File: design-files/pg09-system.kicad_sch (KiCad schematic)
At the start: 34 parts, among them J101 Front Panel, SW201 NMI, SW201 Reset, U101 MC6809E, U102 GAL22V10, U103 74AHCT245, U104 74AHCT245, U105 74AHCT245, U106 GAL22V10, U203 DS1813

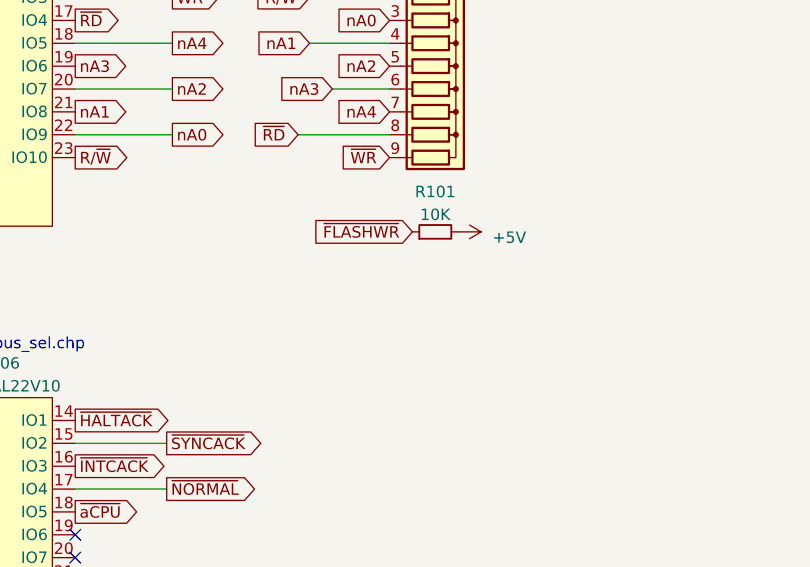
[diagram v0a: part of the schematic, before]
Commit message: Make sure FLASHWREN always has a valid value by pulling it to GND.
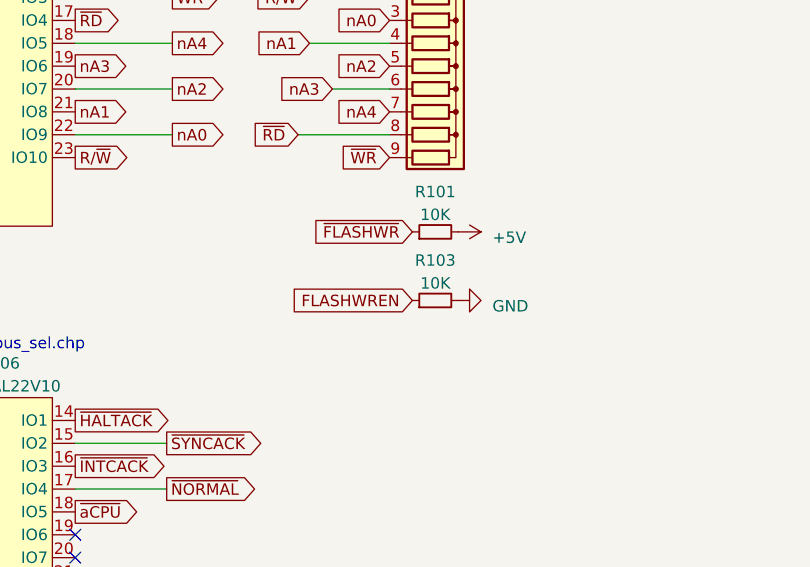
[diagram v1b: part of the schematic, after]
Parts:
- added R103: 10K, Resistor_THT:R_Axial_DIN0207_L6.3mm_D2.5mm_P7.62mm_Horizontal, symbol Device:R_Small
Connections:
- net FLASHWREN: now also R103.1
- net GND: now also R103.2
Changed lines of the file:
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@@
+    )
+  )
+  (global_label "FLASHWREN" (shape input) (at 321.31 163.83 180) (fields_autoplaced)
+    (effects (font (size 1.27 1.27)) (justify right))
+    (property "Intersheetrefs" "${INTERSHEET_REFS}" (at 307.458 163.83 0)
+      (effects (font (size 1.27 1.27)) (justify right) hide)
     )
   )
@@
     )
   )
+  (symbol (lib_id "power:GND") (at 326.39 163.83 90) (unit 1)
+    (in_bom yes) (on_board yes) (dnp no) (fields_autoplaced)
+    (property "Reference" "#PWR0131" (at 332.74 163.83 0)
+      (effects (font (size 1.27 1.27)) hide)
+    )
+    (property "Value" "GND" (at 330.2 164.465 90)
+      (effects (font (size 1.27 1.27)) (justify right))
+    )
+    (property "Footprint" "" (at 326.39 163.83 0)
+      (effects (font (size 1.27 1.27)) hide)
+    )
+    (property "Datasheet" "" (at 326.39 163.83 0)
+      (effects (font (size 1.27 1.27)) hide)
+    )
+    (pin "1")
+    (instances
+      (project "pg09-system"
+        (path "/44572023-3621-4b3a-bd53-c3b2b3f42871"
+          (reference "#PWR0131") (unit 1)
+        )
+      )
+    )
+  )
   (symbol (lib_id "power:GND") (at 116.84 183.388 0) (unit 1)
     (in_bom yes) (on_board yes) (dnp no) (fields_autoplaced)
@@
         )
       )
+    )
+  )
+  (symbol (lib_id "Device:R_Small") (at 323.85 163.83 90) (unit 1)
+    (in_bom yes) (on_board yes) (dnp no) (fields_autoplaced)
+    (property "Reference" "R103" (at 323.85 159.385 90)
+      (effects (font (size 1.27 1.27)))
+    )
+    (property "Value" "10K" (at 323.85 161.925 90)
+      (effects (font (size 1.27 1.27)))
+    )
+    (property "Footprint" "Resistor_THT:R_Axial_DIN0207_L6.3mm_D2.5mm_P7.62mm_Horizontal" (at 323.85 163.83 0)
+      (effects (font (size 1.27 1.27)) hide)
+    )
+    (property "Datasheet" "~" (at 323.85 163.83 0)
+      (effects (font (size 1.27 1.27)) hide)
+    )
+    (pin "1")
+    (pin "2")
+    (instances
+      (project "pg09-system"
+        (path "/44572023-3621-4b3a-bd53-c3b2b3f42871"
+          (reference "R103") (unit 1)
+        )
+      )

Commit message: Revert "Make sure FLASHWREN always has a valid value by pulling it to GND."
This is actually counter-productive due to the internal pull-up on the
GAL inputs.

This reverts commit e5d063032c780da183b0786b1f57988b4be9d05e.
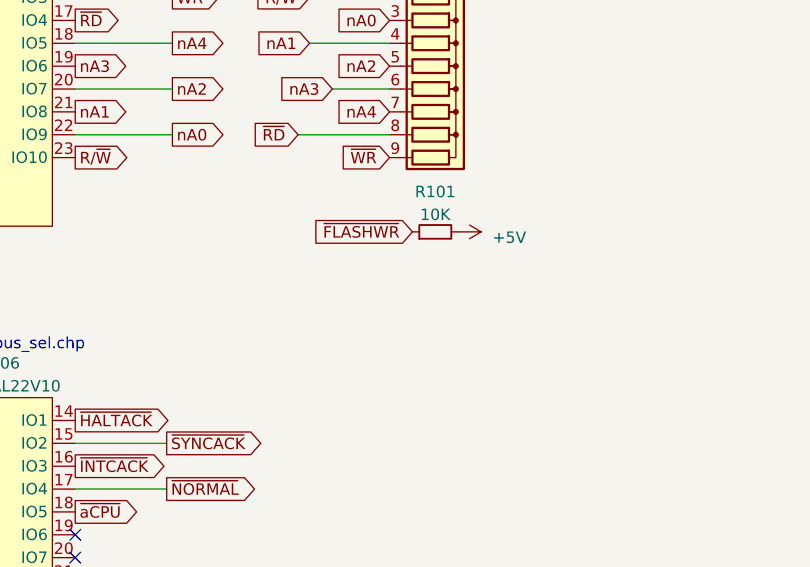
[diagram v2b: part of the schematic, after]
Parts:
- removed R103: 10K, Resistor_THT:R_Axial_DIN0207_L6.3mm_D2.5mm_P7.62mm_Horizontal, symbol Device:R_Small
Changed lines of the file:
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@@
-    )
-  )
-  (global_label "FLASHWREN" (shape input) (at 321.31 163.83 180) (fields_autoplaced)
-    (effects (font (size 1.27 1.27)) (justify right))
-    (property "Intersheetrefs" "${INTERSHEET_REFS}" (at 307.458 163.83 0)
-      (effects (font (size 1.27 1.27)) (justify right) hide)
     )
   )
@@
     )
   )
-  (symbol (lib_id "power:GND") (at 326.39 163.83 90) (unit 1)
-    (in_bom yes) (on_board yes) (dnp no) (fields_autoplaced)
-    (property "Reference" "#PWR0131" (at 332.74 163.83 0)
-      (effects (font (size 1.27 1.27)) hide)
-    )
-    (property "Value" "GND" (at 330.2 164.465 90)
-      (effects (font (size 1.27 1.27)) (justify right))
-    )
-    (property "Footprint" "" (at 326.39 163.83 0)
-      (effects (font (size 1.27 1.27)) hide)
-    )
-    (property "Datasheet" "" (at 326.39 163.83 0)
-      (effects (font (size 1.27 1.27)) hide)
-    )
-    (pin "1")
-    (instances
-      (project "pg09-system"
-        (path "/44572023-3621-4b3a-bd53-c3b2b3f42871"
-          (reference "#PWR0131") (unit 1)
-        )
-      )
-    )
-  )
   (symbol (lib_id "power:GND") (at 116.84 183.388 0) (unit 1)
     (in_bom yes) (on_board yes) (dnp no) (fields_autoplaced)
@@
         )
       )
-    )
-  )
-  (symbol (lib_id "Device:R_Small") (at 323.85 163.83 90) (unit 1)
-    (in_bom yes) (on_board yes) (dnp no) (fields_autoplaced)
-    (property "Reference" "R103" (at 323.85 159.385 90)
-      (effects (font (size 1.27 1.27)))
-    )
-    (property "Value" "10K" (at 323.85 161.925 90)
-      (effects (font (size 1.27 1.27)))
-    )
-    (property "Footprint" "Resistor_THT:R_Axial_DIN0207_L6.3mm_D2.5mm_P7.62mm_Horizontal" (at 323.85 163.83 0)
-      (effects (font (size 1.27 1.27)) hide)
-    )
-    (property "Datasheet" "~" (at 323.85 163.83 0)
-      (effects (font (size 1.27 1.27)) hide)
-    )
-    (pin "1")
-    (pin "2")
-    (instances
-      (project "pg09-system"
-        (path "/44572023-3621-4b3a-bd53-c3b2b3f42871"
-          (reference "R103") (unit 1)
-        )
-      )
